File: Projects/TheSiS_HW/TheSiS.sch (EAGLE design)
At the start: 80 parts, among them IC1 REG1117, IC3 TP4056, IC4 MCP1703CB, IC5 CP2102, K1 G5L, K2 G5L, K3 G5L, T1 DMN3024LSD, U1 ESP-WROOM-32, U2 GY-521MPU6050, X2 ZX62D-B-5PA8

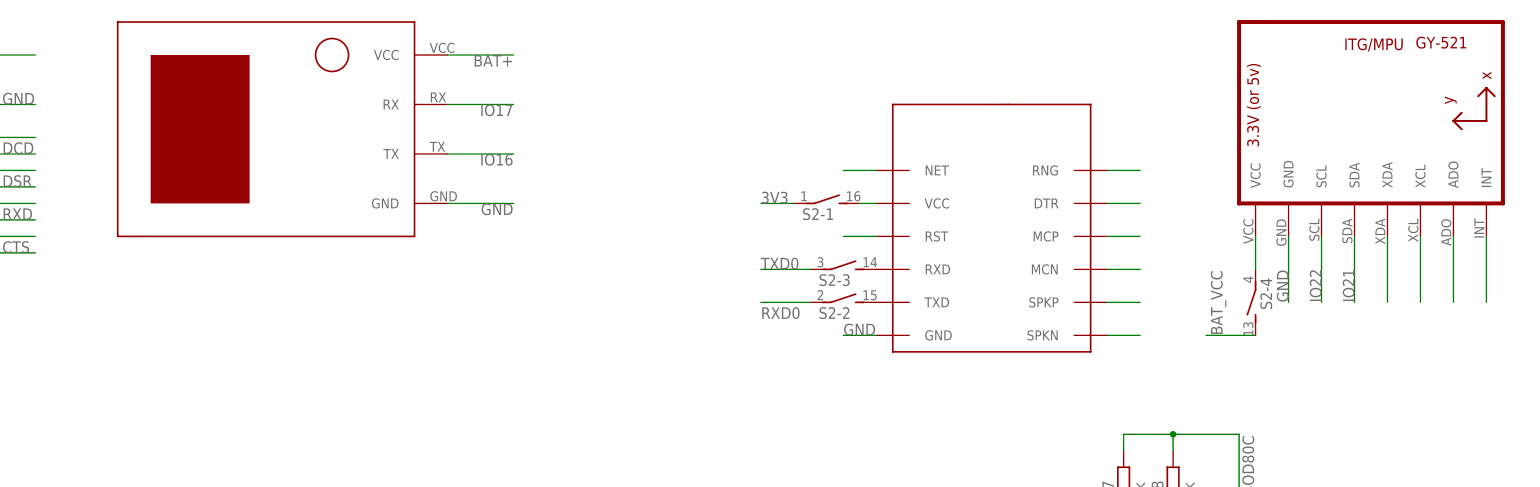
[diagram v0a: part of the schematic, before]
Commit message: Finish Board v20.10.20 [Order PCBWay.com]
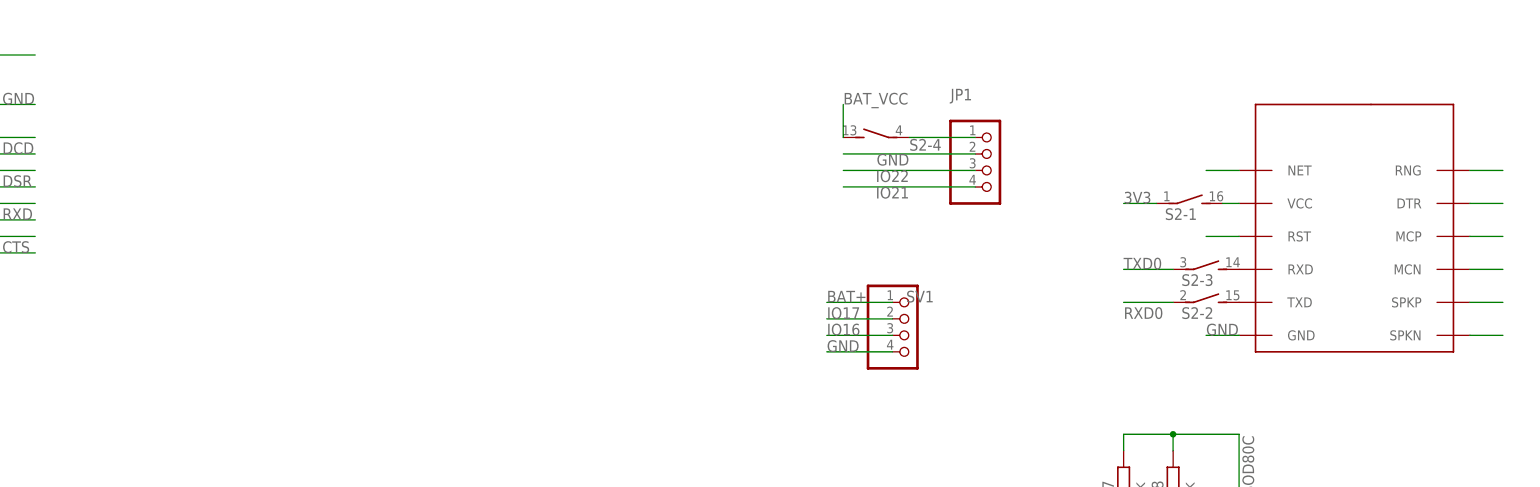
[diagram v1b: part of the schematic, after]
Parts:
- removed U$3: U-BLOX-NEO6V2, u-blox neo-6m v2:U-BLOX-NEO6V2
- removed U2: GY-521MPU6050, gy-521:GY-521MPU6050
- added JP1, SV1: (no value), pinhead:PINHD-1X4
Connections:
- removed net N$33: S2-4.1, U2.VCC
- removed net N$37: U2.XDA
- removed net N$38: U2.XCL
- removed net N$39: U2.ADO
- removed net N$40: U2.INT
- new net N$35: JP1.1, S2-4.1
- net BAT+: now also SV1.1; no longer U$3.VCC
- net GND: now also JP1.2, SV1.4; no longer U$3.GND, U2.GND
- net IO16: now also SV1.3; no longer U$3.TX
- net IO17: now also SV1.2; no longer U$3.RX
- net IO21: now also JP1.4; no longer U2.SDA
- net IO22: now also JP1.3; no longer U2.SCL
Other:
- moved on the sheet: S2-1, S2-2, S2-3, S2-4
